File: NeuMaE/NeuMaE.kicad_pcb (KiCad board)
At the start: 2 copper layers, 52.1 x 53.8 mm, 20 parts, among them J1 MOTOR, J2 PROGRAM, J3 LED, J4 PWR, J5 EXTRA, Q1 BC337, SW1 FLASH, SW2 RESET, U1 PMIC-LD1117V33(TO-220), U2 ESP8266-12E_ESP-12E

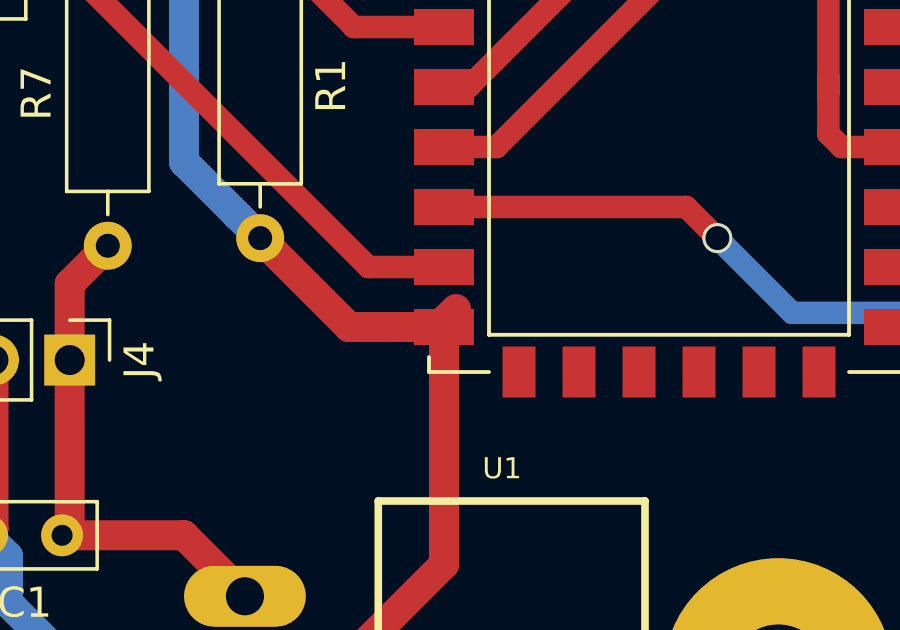
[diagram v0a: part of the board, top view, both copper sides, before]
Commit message: update gerber
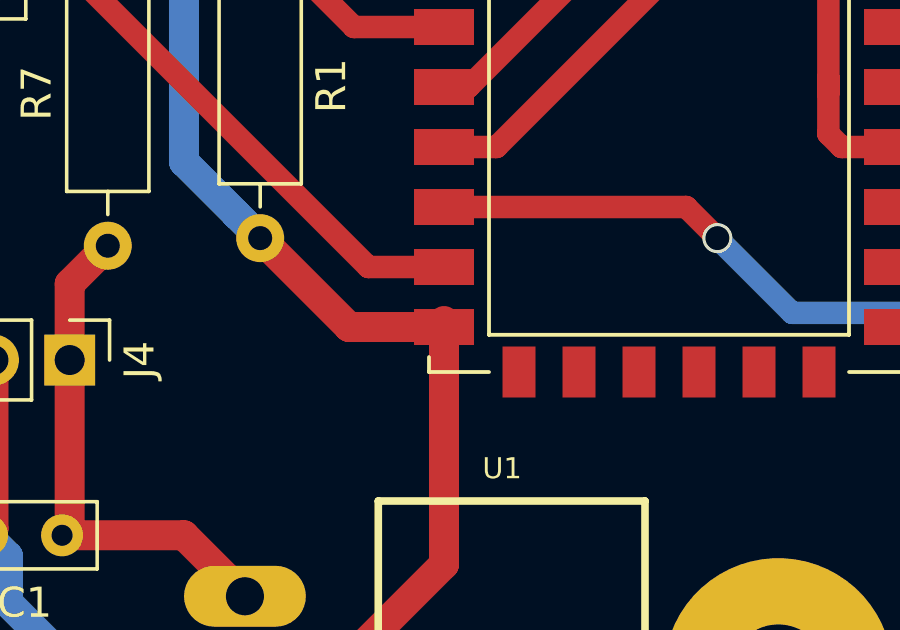
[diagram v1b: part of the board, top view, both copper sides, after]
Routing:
- net +3V3: track 100.7 -> 100.1 mm
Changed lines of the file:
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@@
     (thickness 1.6)
     (drawings 4)
-    (tracks 172)
+    (tracks 171)
     (zones 0)
     (modules 20)
@@
       (outputformat 1)
       (mirror false)
-      (drillshape 1)
+      (drillshape 0)
       (scaleselection 1)
       (outputdirectory ""))
@@
   (segment (start 60.737501 49.775001) (end 60.737501 48.175001) (width 1) (layer F.Cu) (net 5))
   (segment (start 54.102 59.69) (end 55.146225 59.69) (width 1) (layer F.Cu) (net 5))
-  (segment (start 60.737501 47.974499) (end 61.136998 47.575002) (width 1) (layer F.Cu) (net 5))
   (segment (start 60.737501 56.086499) (end 60.737501 47.974499) (width 1) (layer F.Cu) (net 5))
   (segment (start 57.134 59.69) (end 60.737501 56.086499) (width 1) (layer F.Cu) (net 5))
